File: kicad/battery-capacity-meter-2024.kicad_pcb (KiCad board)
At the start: 2 copper layers, 102.5 x 106.6 mm, 77 parts, among them J3 Conn_MainBoard, J4 Conn_DisplayBoard, J5 PWR, Q1 2N3904, Q2 2N3906, Q3 2SD2390, Q6 X0402MF, SW1 CHARGE/DISCHARGE, SW2 1A MODE, U1 LM2596_StepDown_Module, U10 AO3406, U2 LM358, U3 TM1637Display, U5 AO3406, U6 TL431LP, U7 Arduino_pro_mini, U8 TP4056, U9 AO3406

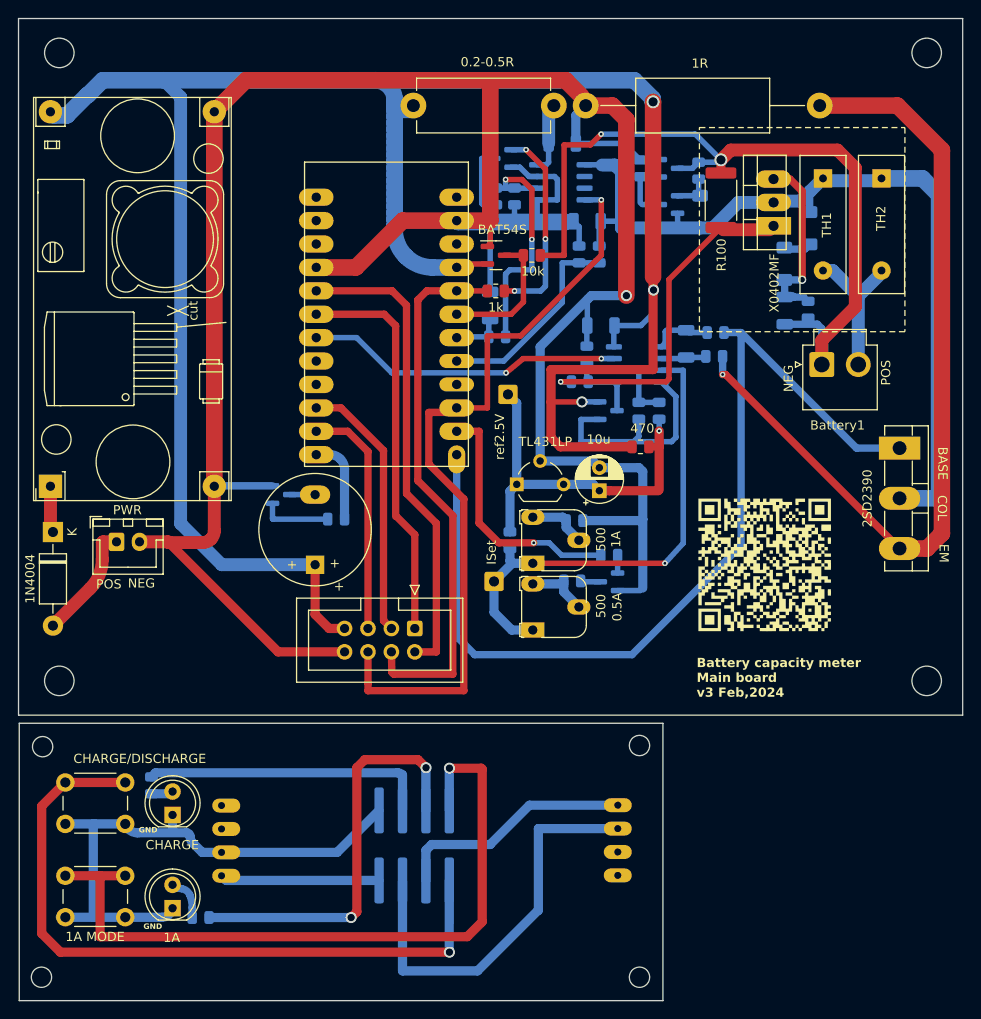
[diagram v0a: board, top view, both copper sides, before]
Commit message: jlc-pcb order
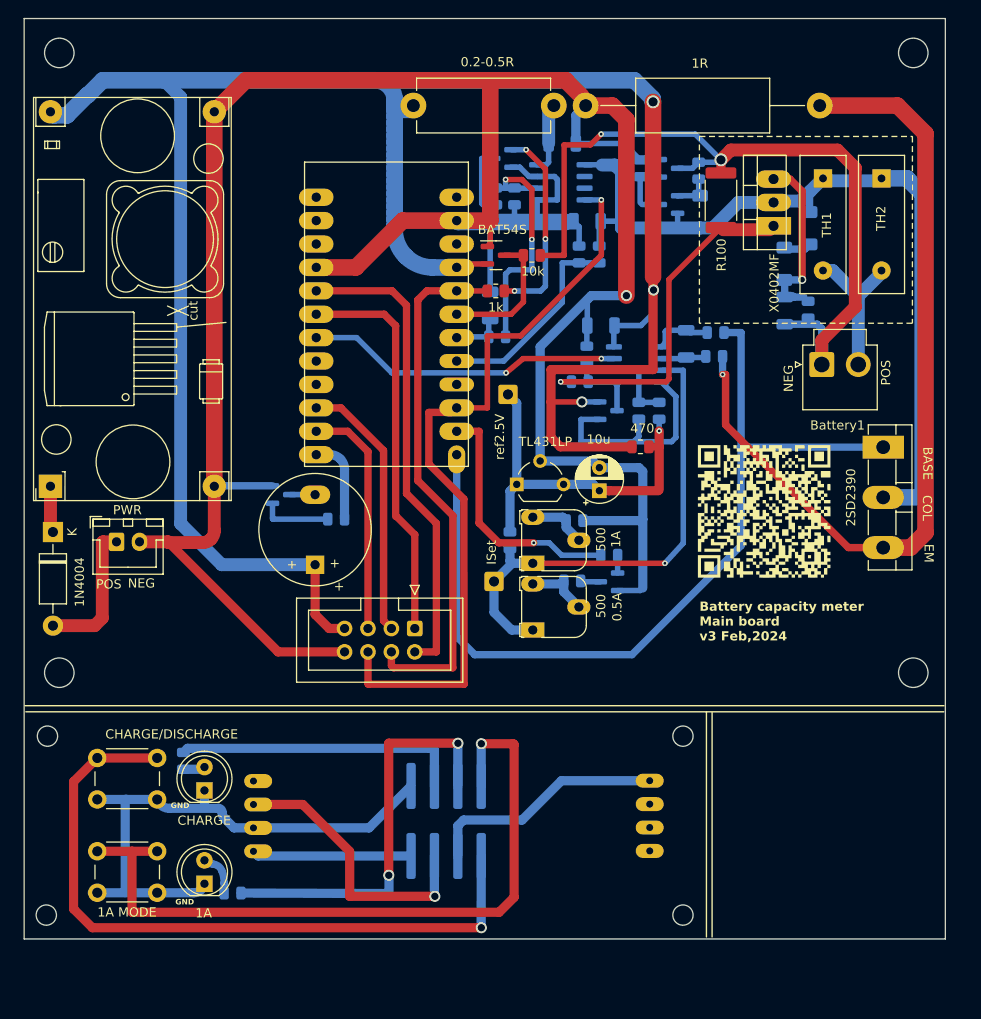
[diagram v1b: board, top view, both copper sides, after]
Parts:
- moved H5 8.23 mm to (167.2, 145.1)
- moved H7 6.77 mm to (98.1, 145.1)
- moved G*** 5.80 mm to (176.1, 101.4)
- moved H6 4.82 mm to (167.2, 125.7)
- moved D3 4.37 mm to (115.2, 131.6)
- moved J4 4.37 mm to (141.5, 134.9)
- moved D4 4.37 mm to (115.2, 141.7)
- moved R19 4.37 mm to (113.0, 128.4)
- moved R20 4.37 mm to (118.3, 142.8)
- moved U3 4.37 mm to (140.1, 132.6)
- moved SW1 4.37 mm to (103.6, 128.1)
- moved SW2 4.37 mm to (103.6, 138.2)
- moved Q3 1.78 mm to (188.9, 94.4)
- moved H2 1.70 mm to (192.2, 118.8)
- moved H1 1.46 mm to (192.2, 51.6)
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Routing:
- net DIO: track 70.5 -> 56.9 mm, vias 0 -> 1
- net DSCHRG_EN: track 103.7 -> 96.7 mm
- net Net-(D1-A): track 12.6 -> 15.5 mm
- net 1A_MODE: track 103.8 -> 102.2 mm
- net CHRG_EN: track 115.2 -> 113.8 mm
- net Net-(D2-K): track 93.8 -> 92.6 mm
- net Net-(Q3-E): track 91.1 -> 91.7 mm
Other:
- board size 102.5 x 106.6 mm -> 100 x 99.9 mm
